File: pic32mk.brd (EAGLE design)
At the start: 100 x 80 mm, 73 parts, among them IC1 PIC32MK1024MCF100-I_PT, IC2 ADM3095EBRZ, IC3 TXB0101DCKR, IC4 MAX203ECWP, IC5 TXB0101DCKR, IC6 TXB0101DCKR, IC7 TXB0101DCKR, IC8 TXB0101DCKR, IC9 TXB0101DCKR, J1 1-1586043-4, U1 PMIC-MC33932VW(SOP44), U2 PMIC-MC33932VW(SOP44), X1 22-23-2101, X3 22-23-2101

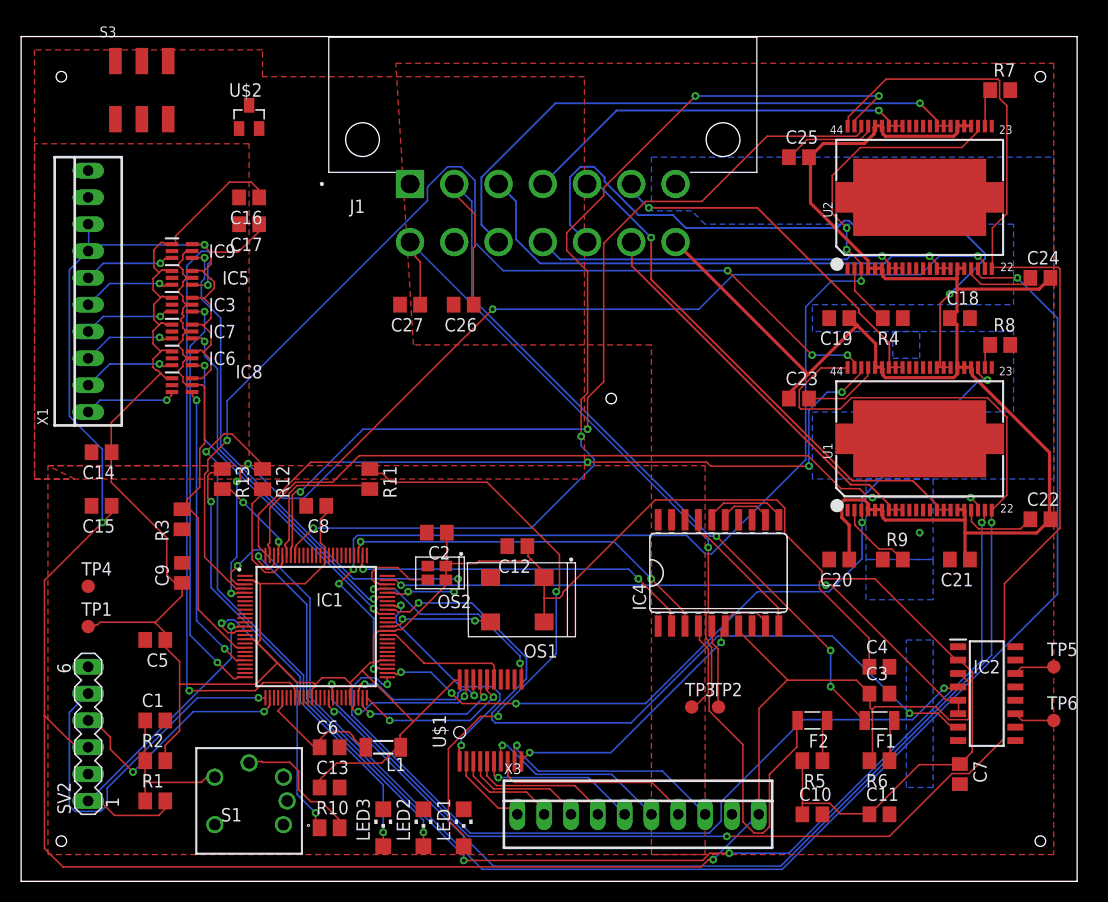
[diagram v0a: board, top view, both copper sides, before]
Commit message: up
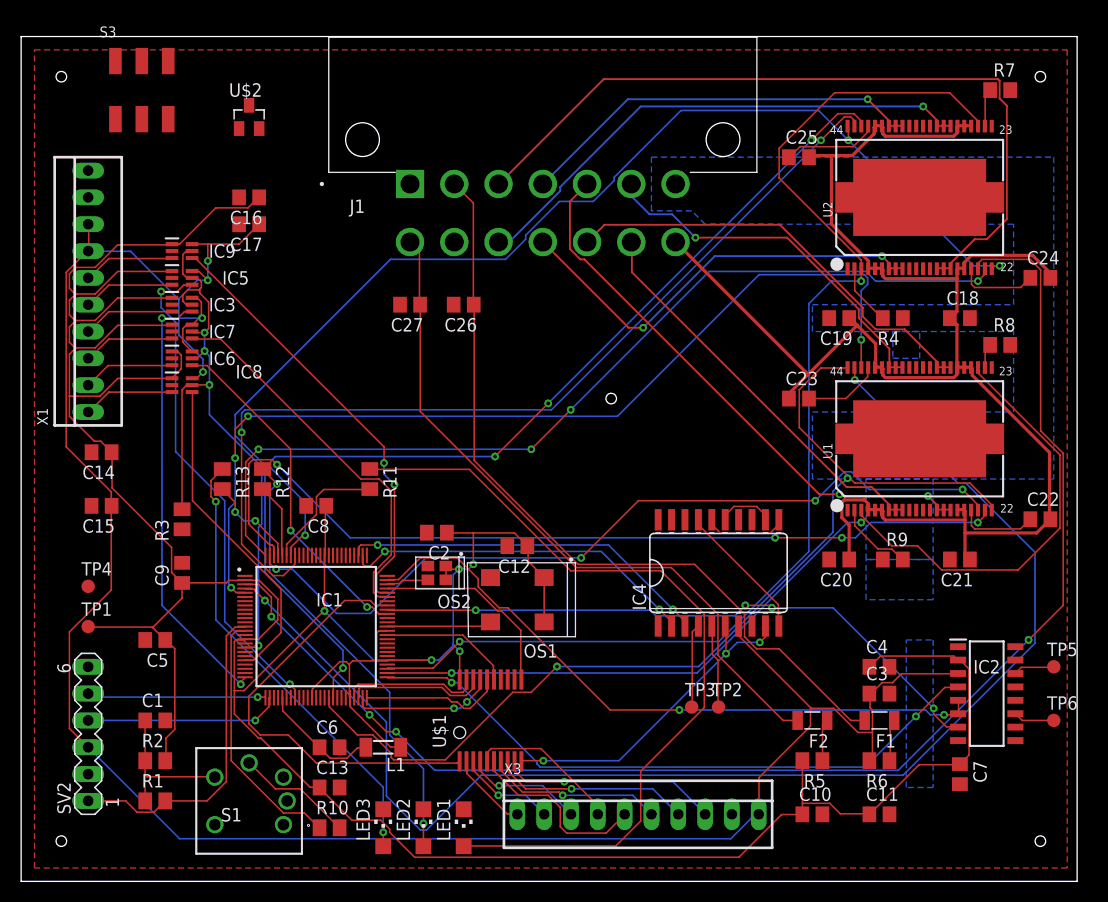
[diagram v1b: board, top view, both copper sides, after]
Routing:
- net VDD: track 289.1 -> 351.6 mm, vias 0 -> 5
- net U2FS: track 164.4 -> 124.5 mm, vias 2 -> 3
- net U1FS: track 129.4 -> 96.5 mm
- net PWM1H: track 101.8 -> 129.4 mm, vias 4 -> 2
- net PWM2H: track 111.4 -> 84.1 mm
- net U204: track 49.2 -> 74.0 mm, vias 1 -> 0
- net U1O3: track 64.6 -> 41.6 mm, vias 1 -> 0
- net +3V3: track 89.1 -> 66.6 mm, vias 1 -> 0
- net N$36: track 54.9 -> 77.2 mm, vias 2 -> 0
- net VCC: track 232.0 -> 213.2 mm, vias 3 -> 4
- net N$14: track 35.5 -> 16.9 mm
- net RD8: track 23.9 -> 41.2 mm, vias 2 -> 0
- net RPE0: track 77.2 -> 92.8 mm, vias 5 -> 2
- net U6TX: track 76.1 -> 60.8 mm
- net U6RX: track 74.2 -> 59.8 mm, vias 2 -> 4
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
